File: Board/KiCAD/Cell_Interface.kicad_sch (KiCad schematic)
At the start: 26 parts, among them Q23 2N7002, Q24 2N7002, Q25 2N7002, Q26 2N7002, Q5 BSS83P, Q6 BSS83P, Q7 BSS83P, Q8 BSS83P, U6 INA219AxDCN, U7 INA219AxDCN, U8 INA219AxDCN

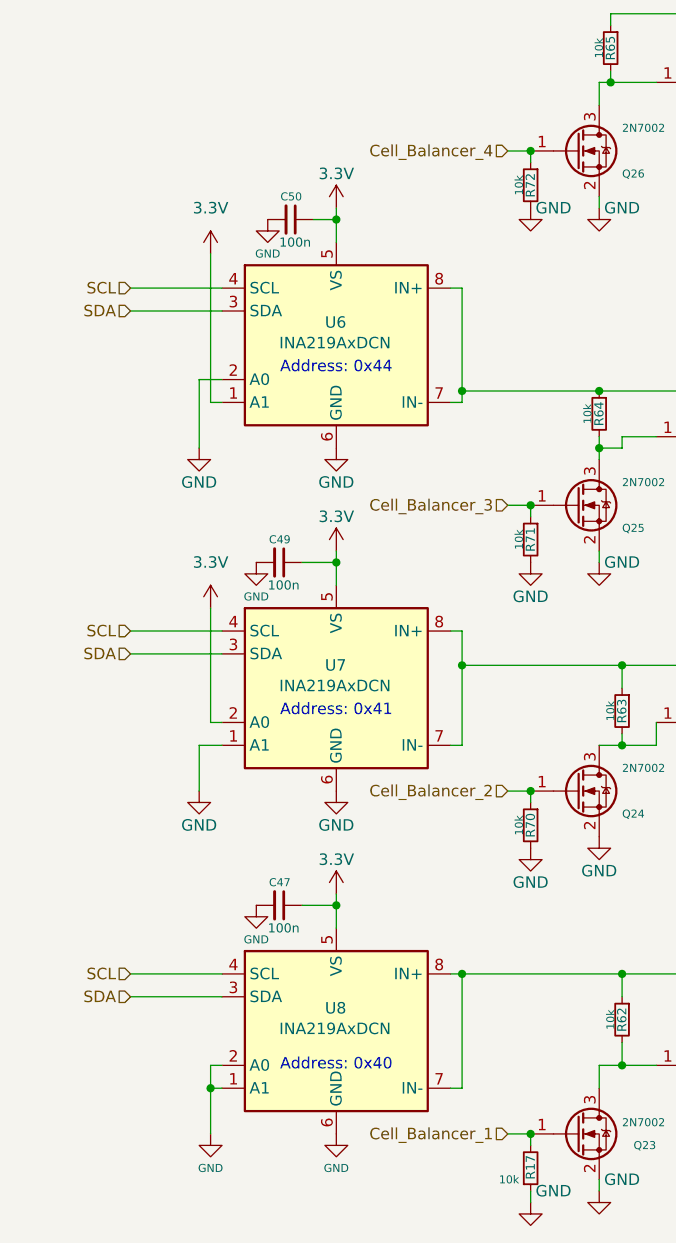
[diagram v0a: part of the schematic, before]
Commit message: PCB Revision
PCN near full completion, currently running on no errors while running DRC.

@KeytarGoblin @andrewgreenberg @Danish2PSU
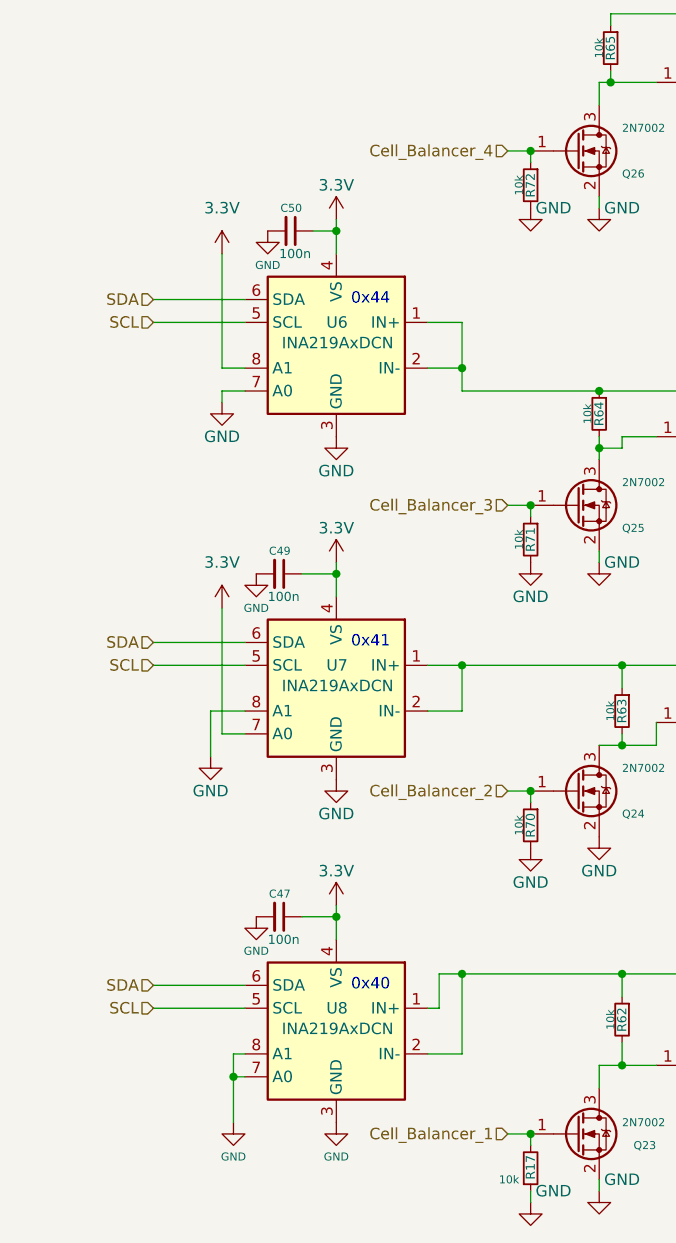
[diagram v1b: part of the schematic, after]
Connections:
- net 3.3V: now also U6.4 (VS), U6.8 (A1), U7.4 (VS), U7.7 (A0), U8.4 (VS); no longer U6.1 (A1), U6.5 (VS), U7.2 (A0), U7.5 (VS), U8.5 (VS)
- net Cell 1: now also U8.1 (IN+), U8.2 (IN-); no longer U8.7 (IN-), U8.8 (IN+)
- net Cell 2: now also U7.1 (IN+), U7.2 (IN-); no longer U7.7 (IN-), U7.8 (IN+)
- net Cell 3: now also U6.1 (IN+), U6.2 (IN-); no longer U6.7 (IN-), U6.8 (IN+)
- net GND: now also U6.3 (GND), U6.7 (A0), U7.3 (GND), U7.8 (A1), U8.3 (GND), U8.7 (A0), U8.8 (A1); no longer U6.2 (A0), U6.6 (GND), U7.1 (A1), U7.6 (GND), U8.1 (A1), U8.2 (A0), U8.6 (GND)
- net SCL: now also U6.5 (SCL), U7.5 (SCL), U8.5 (SCL); no longer U6.4 (SCL), U7.4 (SCL), U8.4 (SCL)
- net SDA: now also U6.6 (SDA), U7.6 (SDA), U8.6 (SDA); no longer U6.3 (SDA), U7.3 (SDA), U8.3 (SDA)
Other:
- note added: "0x40"
- note added: "0x41"
- note added: "0x44"
- note removed: "Address: 0x40"
- note removed: "Address: 0x41"
- note removed: "Address: 0x44"
- moved on the sheet: C47, C49, C50
